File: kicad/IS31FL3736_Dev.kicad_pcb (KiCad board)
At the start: 4 copper layers, 70.7 x 31.5 mm, 57 parts, among them J1 Daisy IN, J2 Daisy OUT, U1 IS31FL3736

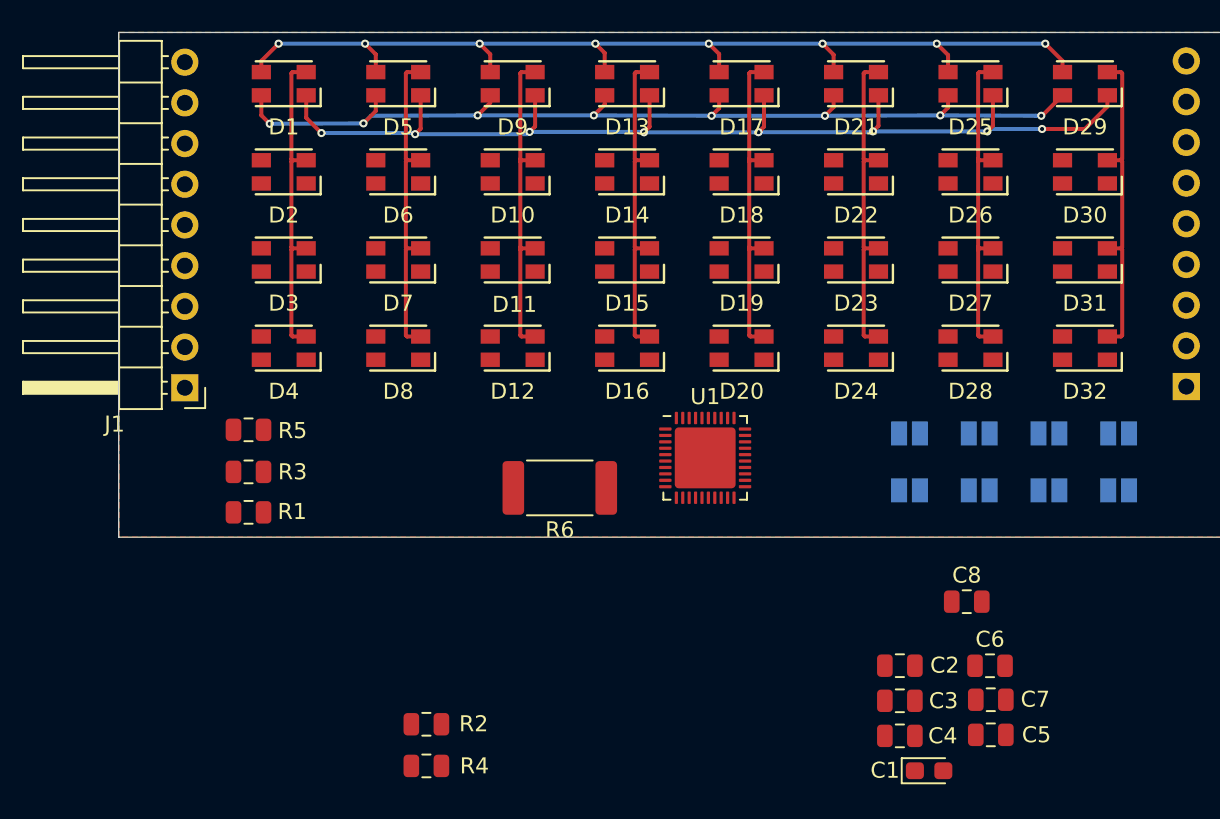
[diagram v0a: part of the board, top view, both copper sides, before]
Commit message: Board update
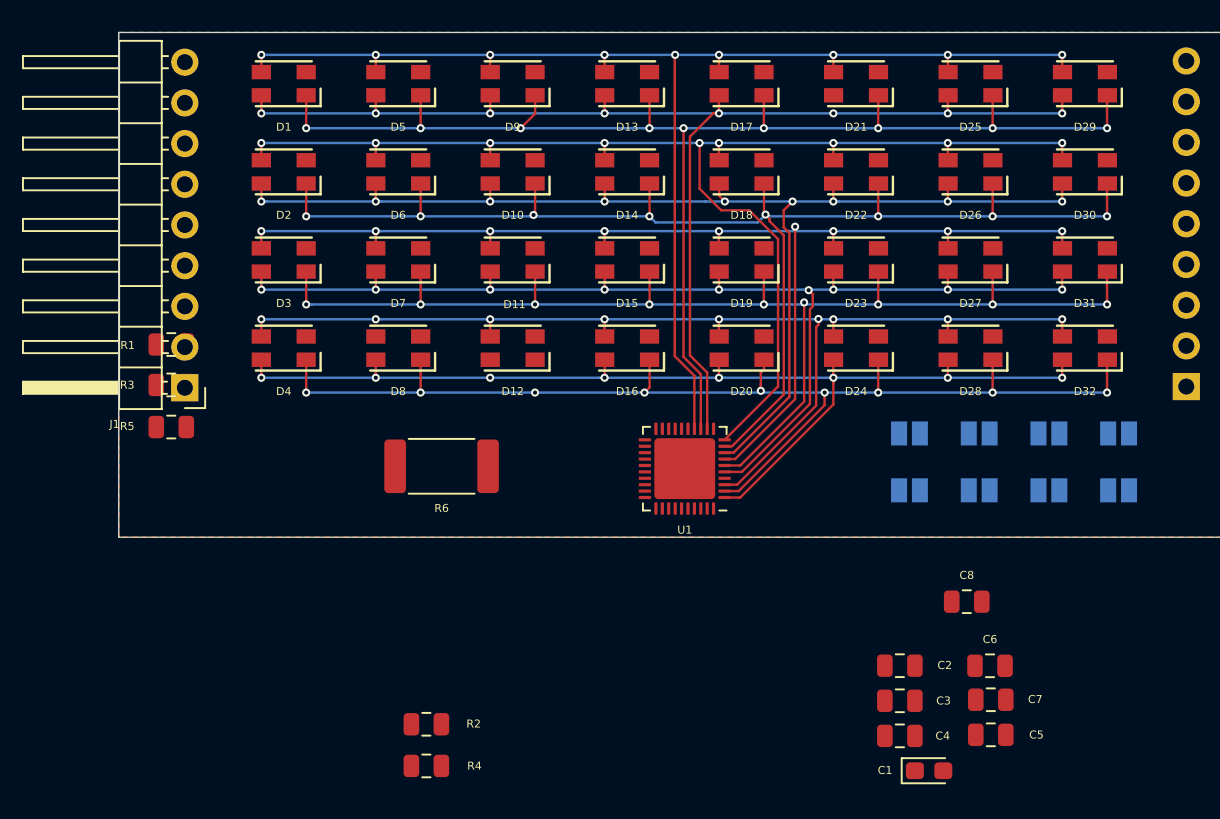
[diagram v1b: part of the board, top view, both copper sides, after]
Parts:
- moved R1 11.5 mm to (130.4, 133.6), turned to 180 degrees
- moved R6 7.50 mm to (147.2, 141.2)
- moved R3 7.26 mm to (130.4, 136.1), turned to 180 degrees
- moved R5 4.82 mm to (130.4, 138.7), turned to 180 degrees
- moved U1 1.44 mm to (162.4, 141.3), turned to 180 degrees
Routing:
- net /SW8: track 0.00 -> 83.4 mm, vias 0 -> 8
- net /SW9: track 0.00 -> 81.6 mm, vias 0 -> 9
- net /SW5: track 0.00 -> 79.3 mm, vias 0 -> 9
- net /SW7: track 0.00 -> 77.5 mm, vias 0 -> 9
- net /SW6: track 0.00 -> 75.3 mm, vias 0 -> 9
- net /SW2: track 0.00 -> 73.8 mm, vias 0 -> 9
- net /SW4: track 0.00 -> 73.4 mm, vias 0 -> 9
- net /SW3: track 0.00 -> 70.8 mm, vias 0 -> 9
- net /SW1: track 0.00 -> 68.7 mm, vias 0 -> 8
- net /CS8: track 20.3 -> 0.00 mm
- net /CS6: track 20.1 -> 0.00 mm
- net /CS3: track 20.1 -> 0.00 mm
- net /CS2: track 20.1 -> 0.00 mm
- net /CS5: track 20.1 -> 0.00 mm
- net /CS1: track 20.1 -> 0.00 mm
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
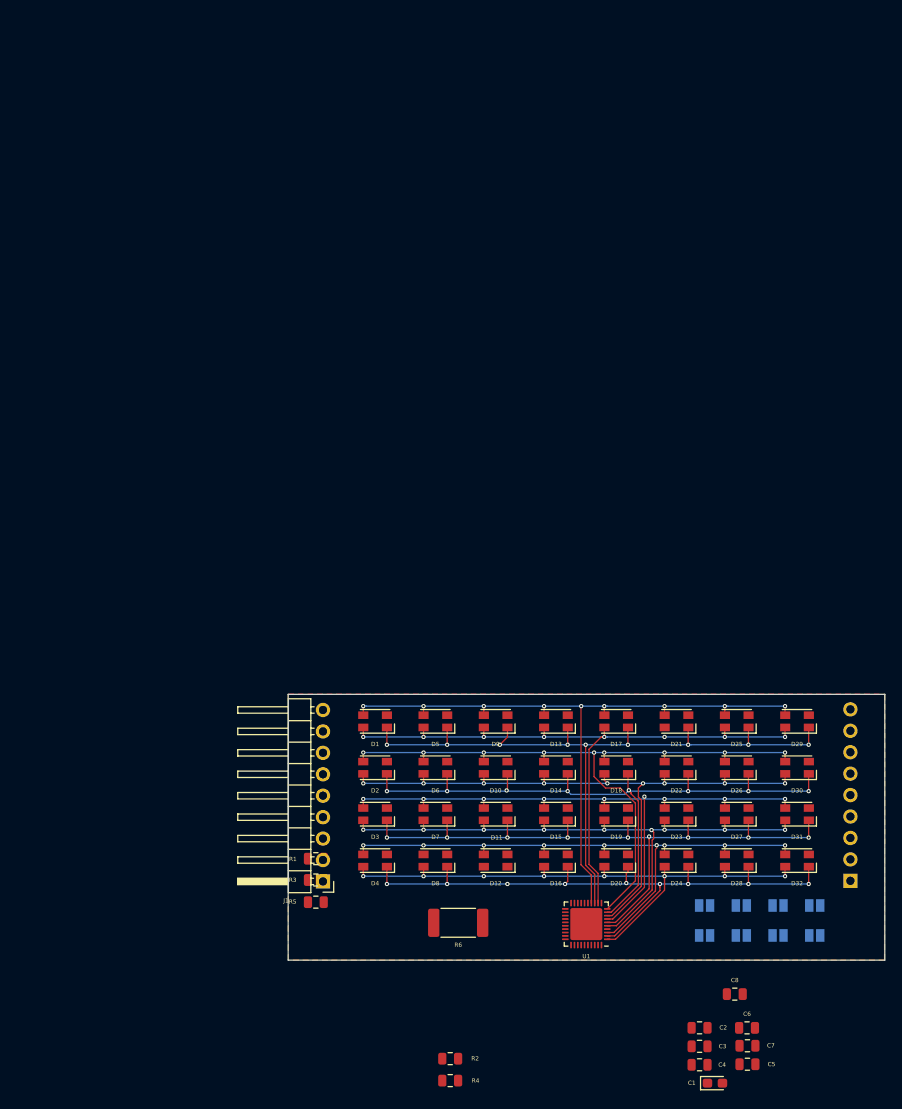
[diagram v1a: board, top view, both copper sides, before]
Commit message: Layout done
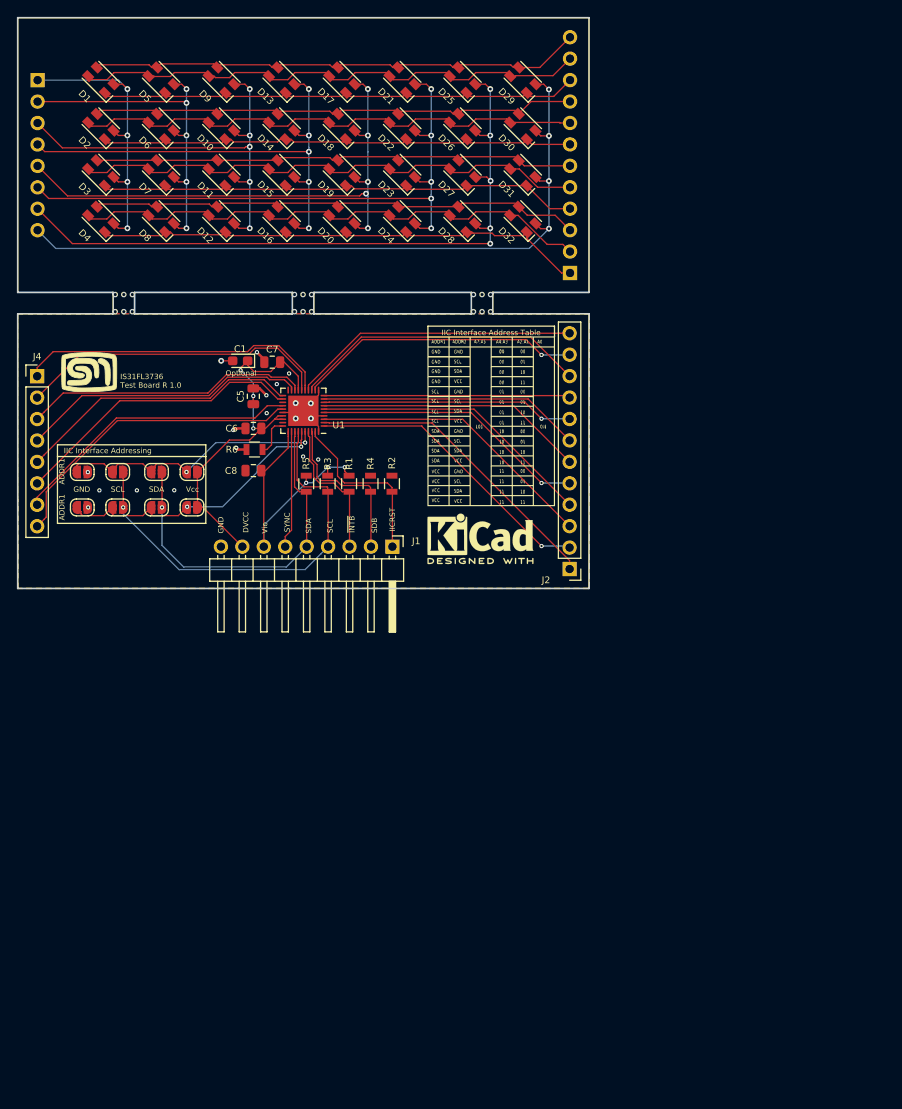
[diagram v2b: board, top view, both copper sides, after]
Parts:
- removed C2, C3, C4: 0.47μF, Capacitor_SMD:C_0805_2012Metric
- added G***: LOGO, is31fl3736_dev:Address_Table, F.Cu at (151.1, 81.7)
- added G***: LOGO, is31fl3736_dev:MyBasic_rounded_50_1, F.Cu at (103.5, 75.9)
- added J3: Top_SW_Connector, Pin_Headers:Pin_Header_Straight_1x12_Pitch2.54mm, B.Cu at (160.5, 64.2)
- added J4: Bottom_CS_Connector, Pin_Headers:Pin_Header_Straight_1x08_Pitch2.54mm, F.Cu at (97.3, 76.4)
- added J5: Top_CS_Connector, Pin_Headers:Pin_Header_Straight_1x08_Pitch2.54mm, B.Cu at (97.4, 41.3)
- added REF**: MouseBites, is31fl3736_dev:MouseBites, F.Cu at (148.8, 69.0)
- added REF**: MouseBites, is31fl3736_dev:MouseBites, F.Cu at (127.6, 69.0)
- added REF**: MouseBites, is31fl3736_dev:MouseBites, F.Cu at (106.3, 69.0)
- added REF***: KiCad-Logo2_6mm_SilkScreen, Symbols:KiCad-Logo2_6mm_SilkScreen, F.Cu at (149.9, 95.7)
- J2: value Daisy OUT -> Bottom_SW_Connector; footprint Connector_PinHeader_2.54mm:PinHeader_1x09_P2.54mm_Horizontal -> Pin_Headers:Pin_Header_Straight_1x12_Pitch2.54mm; moved to F.Cu
- JP1, JP2, JP3, JP4, JP5, JP6, JP8: footprint Jumper:SolderJumper-2_P1.3mm_Open_Pad1.0x1.5mm -> Jumper:SolderJumper-2_P1.3mm_Open_RoundedPad1.0x1.5mm; moved to F.Cu
- JP7: value SLC ADDR2 -> SCL ADDR2; footprint Jumper:SolderJumper-2_P1.3mm_Open_Pad1.0x1.5mm -> Jumper:SolderJumper-2_P1.3mm_Open_RoundedPad1.0x1.5mm; moved to F.Cu
- R1, R2, R3, R4, R5: footprint Resistor_SMD:R_0805_2012Metric -> Resistors_SMD:R_0805
- R6: footprint Resistor_SMD:R_2512_6332Metric -> Resistors_SMD:R_0805
- U1: footprint Package_DFN_QFN:QFN-40-1EP_5x5mm_P0.4mm_EP3.8x3.8mm -> Housings_DFN_QFN:QFN-40-1EP_5x5mm_Pitch0.4mm
- moved C1 102.4 mm to (121.4, 74.6), turned to 180 degrees
- moved JP8 100.9 mm to (102.7, 87.8), turned to 180 degrees
- moved JP7 99.2 mm to (106.9, 87.8), turned to 180 degrees
- moved C7 98.7 mm to (125.2, 74.7), turned to 180 degrees
- moved C5 98.5 mm to (123.0, 78.8), turned to 90 degrees
- moved C6 92.0 mm to (123.0, 82.6), turned to 180 degrees
- moved JP4 91.2 mm to (102.7, 92.0), turned to 180 degrees
- moved JP6 89.8 mm to (111.5, 87.8), turned to 180 degrees
- moved JP3 89.6 mm to (106.9, 92.0), turned to 180 degrees
- moved JP5 88.5 mm to (115.7, 87.8), turned to 180 degrees
- moved C8 84.3 mm to (123.0, 87.6), turned to 180 degrees
- moved D15 82.6 mm to (126.3, 52.3), turned to 315 degrees
- moved D16 82.6 mm to (126.3, 57.8), turned to 315 degrees
- moved D19 82.6 mm to (133.5, 52.3), turned to 315 degrees
- moved D20 82.6 mm to (133.5, 57.8), turned to 315 degrees
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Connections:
- D1 pad 1: /SW11 -> /TSW11
- D1 pad 2: /SW10 -> /TSW10
- D1 pad 3: /SW12 -> /TSW12
- D1 pad 4: /CS1 -> /TCS1
- D10 pad 1: /SW8 -> /TSW8
- D10 pad 2: /SW7 -> /TSW7
- D10 pad 3: /SW9 -> /TSW9
- D10 pad 4: /CS3 -> /TCS3
- D11 pad 1: /SW5 -> /TSW5
- D11 pad 2: /SW4 -> /TSW4
- D11 pad 3: /SW6 -> /TSW6
- D11 pad 4: /CS3 -> /TCS3
- D12 pad 1: /SW2 -> /TSW2
- D12 pad 2: /SW1 -> /TSW1
- D12 pad 3: /SW3 -> /TSW3
- D12 pad 4: /CS3 -> /TCS3
- D13 pad 1: /SW11 -> /TSW11
- D13 pad 2: /SW10 -> /TSW10
- D13 pad 3: /SW12 -> /TSW12
- D13 pad 4: /CS4 -> /TCS4
- D14 pad 1: /SW8 -> /TSW8
- D14 pad 2: /SW7 -> /TSW7
- D14 pad 3: /SW9 -> /TSW9
- D14 pad 4: /CS4 -> /TCS4
- D15 pad 1: /SW5 -> /TSW5
- D15 pad 2: /SW4 -> /TSW4
- D15 pad 3: /SW6 -> /TSW6
- D15 pad 4: /CS4 -> /TCS4
- D16 pad 1: /SW2 -> /TSW2
- D16 pad 2: /SW1 -> /TSW1
- D16 pad 3: /SW3 -> /TSW3
- D16 pad 4: /CS4 -> /TCS4
- D17 pad 1: /SW11 -> /TSW11
- D17 pad 2: /SW10 -> /TSW10
- D17 pad 3: /SW12 -> /TSW12
- D17 pad 4: /CS5 -> /TCS5
- D18 pad 1: /SW8 -> /TSW8
- D18 pad 2: /SW7 -> /TSW7
- D18 pad 3: /SW9 -> /TSW9
- D18 pad 4: /CS5 -> /TCS5
- D19 pad 1: /SW5 -> /TSW5
- D19 pad 2: /SW4 -> /TSW4
- D19 pad 3: /SW6 -> /TSW6
- D19 pad 4: /CS5 -> /TCS5
- D2 pad 1: /SW8 -> /TSW8
- D2 pad 2: /SW7 -> /TSW7
- D2 pad 3: /SW9 -> /TSW9
- D2 pad 4: /CS1 -> /TCS1
- D20 pad 1: /SW2 -> /TSW2
- D20 pad 2: /SW1 -> /TSW1
- D20 pad 3: /SW3 -> /TSW3
- D20 pad 4: /CS5 -> /TCS5
- D21 pad 1: /SW11 -> /TSW11
- D21 pad 2: /SW10 -> /TSW10
- D21 pad 3: /SW12 -> /TSW12
- D21 pad 4: /CS6 -> /TCS6
- D22 pad 1: /SW8 -> /TSW8
- D22 pad 2: /SW7 -> /TSW7
- D22 pad 3: /SW9 -> /TSW9
- D22 pad 4: /CS6 -> /TCS6
- D23 pad 1: /SW5 -> /TSW5
- D23 pad 2: /SW4 -> /TSW4
- D23 pad 3: /SW6 -> /TSW6
- D23 pad 4: /CS6 -> /TCS6
- D24 pad 1: /SW2 -> /TSW2
- D24 pad 2: /SW1 -> /TSW1
- D24 pad 3: /SW3 -> /TSW3
- D24 pad 4: /CS6 -> /TCS6
- D25 pad 1: /SW11 -> /TSW11
- D25 pad 2: /SW10 -> /TSW10
- D25 pad 3: /SW12 -> /TSW12
- D25 pad 4: /CS7 -> /TCS7
- D26 pad 1: /SW8 -> /TSW8
- D26 pad 2: /SW7 -> /TSW7
- D26 pad 3: /SW9 -> /TSW9
- D26 pad 4: /CS7 -> /TCS7
- D27 pad 1: /SW5 -> /TSW5
- D27 pad 2: /SW4 -> /TSW4
- D27 pad 3: /SW6 -> /TSW6
- D27 pad 4: /CS7 -> /TCS7
- D28 pad 1: /SW2 -> /TSW2
- D28 pad 2: /SW1 -> /TSW1
- D28 pad 3: /SW3 -> /TSW3
- D28 pad 4: /CS7 -> /TCS7
- D29 pad 1: /SW11 -> /TSW11
- D29 pad 2: /SW10 -> /TSW10
- D29 pad 3: /SW12 -> /TSW12
- D29 pad 4: /CS8 -> /TCS8
- D3 pad 1: /SW5 -> /TSW5
- D3 pad 2: /SW4 -> /TSW4
- D3 pad 3: /SW6 -> /TSW6
- D3 pad 4: /CS1 -> /TCS1
- D30 pad 1: /SW8 -> /TSW8
- D30 pad 2: /SW7 -> /TSW7
- D30 pad 3: /SW9 -> /TSW9
- D30 pad 4: /CS8 -> /TCS8
- D31 pad 1: /SW5 -> /TSW5
- D31 pad 2: /SW4 -> /TSW4
- D31 pad 3: /SW6 -> /TSW6
- D31 pad 4: /CS8 -> /TCS8
- D32 pad 1: /SW2 -> /TSW2
- D32 pad 2: /SW1 -> /TSW1
- D32 pad 3: /SW3 -> /TSW3
- D32 pad 4: /CS8 -> /TCS8
- D4 pad 1: /SW2 -> /TSW2
- D4 pad 2: /SW1 -> /TSW1
- D4 pad 3: /SW3 -> /TSW3
- D4 pad 4: /CS1 -> /TCS1
- D5 pad 1: /SW11 -> /TSW11
- D5 pad 2: /SW10 -> /TSW10
- D5 pad 3: /SW12 -> /TSW12
- D5 pad 4: /CS2 -> /TCS2
- D6 pad 1: /SW8 -> /TSW8
- D6 pad 2: /SW7 -> /TSW7
- D6 pad 3: /SW9 -> /TSW9
- D6 pad 4: /CS2 -> /TCS2
- D7 pad 1: /SW5 -> /TSW5
- D7 pad 2: /SW4 -> /TSW4
- D7 pad 3: /SW6 -> /TSW6
- D7 pad 4: /CS2 -> /TCS2
- D8 pad 1: /SW2 -> /TSW2
- D8 pad 2: /SW1 -> /TSW1
- D8 pad 3: /SW3 -> /TSW3
- D8 pad 4: /CS2 -> /TCS2
- D9 pad 1: /SW11 -> /TSW11
- D9 pad 2: /SW10 -> /TSW10
- D9 pad 3: /SW12 -> /TSW12
- D9 pad 4: /CS3 -> /TCS3
- J1 pad 1: /DVCC -> /IICRST
- J1 pad 2: /Vio -> /~SDB
- J1 pad 3: /SDA -> /~INT_B
- J1 pad 5: /~INT_B -> /SDA
- J1 pad 6: /~SDB -> /SYNC
- J1 pad 7: /SYNC -> /Vio
- J1 pad 8: /IICRST -> /DVCC
- J2 pad 1: /DVCC -> /BSW2
- J2 pad 2: /Vio -> /BSW1
- J2 pad 3: /SDA -> /BSW3
- J2 pad 4: /SCL -> /BSW5
- J2 pad 5: /~INT_B -> /BSW4
- J2 pad 6: /~SDB -> /BSW6
- J2 pad 7: /SYNC -> /BSW8
- J2 pad 8: /IICRST -> /BSW7
- J2 pad 9: GND -> /BSW9
- R4 pad 2: /IICRST -> /~SDB
- U1 pad 1: /SW1 -> /BSW1
- U1 pad 10: /SW9 -> /BSW9
- U1 pad 12: /SW10 -> /BSW10
- U1 pad 13: /SW11 -> /BSW11
- U1 pad 14: /SW12 -> /BSW12
- U1 pad 15: /CS1 -> /BCS1
- U1 pad 16: /CS2 -> /BCS2
- U1 pad 18: /CS3 -> /BCS3
- U1 pad 19: /CS4 -> /BCS4
- U1 pad 2: /SW2 -> /BSW2
- U1 pad 21: /CS5 -> /BCS5
- U1 pad 22: /CS6 -> /BCS6
- U1 pad 24: /CS7 -> /BCS7
- U1 pad 25: /CS8 -> /BCS8
- U1 pad 3: /SW3 -> /BSW3
- U1 pad 5: /SW4 -> /BSW4
- U1 pad 6: /SW5 -> /BSW5
- U1 pad 7: /SW6 -> /BSW6
- U1 pad 8: /SW7 -> /BSW7
- U1 pad 9: /SW8 -> /BSW8
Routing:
- net /TCS8: track 0.00 -> 86.3 mm, vias 0 -> 4
- net /SW11: track 86.0 -> 0.00 mm, vias 9 -> 0
- net /SW8: track 83.4 -> 0.00 mm, vias 8 -> 0
- net /SW12: track 82.5 -> 0.00 mm, vias 9 -> 0
- net /TCS7: track 0.00 -> 81.8 mm, vias 0 -> 5
- net /SW9: track 81.6 -> 0.00 mm, vias 9 -> 0
- net /SW5: track 79.3 -> 0.00 mm, vias 9 -> 0
- net /SW10: track 79.0 -> 0.00 mm, vias 8 -> 0
- net /SW7: track 77.5 -> 0.00 mm, vias 9 -> 0
- net /SW6: track 75.3 -> 0.00 mm, vias 9 -> 0
- net /SW2: track 73.8 -> 0.00 mm, vias 9 -> 0
- net /SW4: track 73.4 -> 0.00 mm, vias 9 -> 0
- net /TCS6: track 0.00 -> 72.4 mm, vias 0 -> 5
- net /SW3: track 70.8 -> 0.00 mm, vias 9 -> 0
- net /SW1: track 68.7 -> 0.00 mm, vias 8 -> 0
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- added copper zone on B.Cu, net GND
- removed copper zone on In2.Cu, net /Vio
- removed copper zone on In1.Cu, net GND
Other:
- board size 70.7 x 31.5 mm -> 67.7 x 67.6 mm
- copper layers 4 -> 2
- net class Default: clearance 0.2 -> 0.1524; trace_width 0.25 -> 0.1524; via_dia 0.8 -> 0.6858; via_drill 0.4 -> 0.3302
- net class LED added: clearance 0.1524, trace_width 0.1524, via_dia 0.508, via_drill 0.254
- rule pad_to_mask_clearance: 0.0508 -> 0
- rule trace_clearance: 0.2 -> 0.1524
- board text added: "ADDR1"
- board text added: "DVCC"
- board text added: "GND"
- board text added: "IIC Interface Address Table"
- board text added: "IIC Interface Addressing"
- board text added: "IICRST"
- board text added: "IS31FL3736 Test Board R 1.0"
- board text added: "Optional"
- board text added: "SCL"
- board text added: "SDA"
- board text added: "SDB"
- board text added: "SYNC"
- board text added: "Vcc"
- board text added: "Vio"
- board text added: "~INTB"
